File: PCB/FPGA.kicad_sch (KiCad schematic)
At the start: 1 part, among them U1 LFE5U-25F-6BG256C

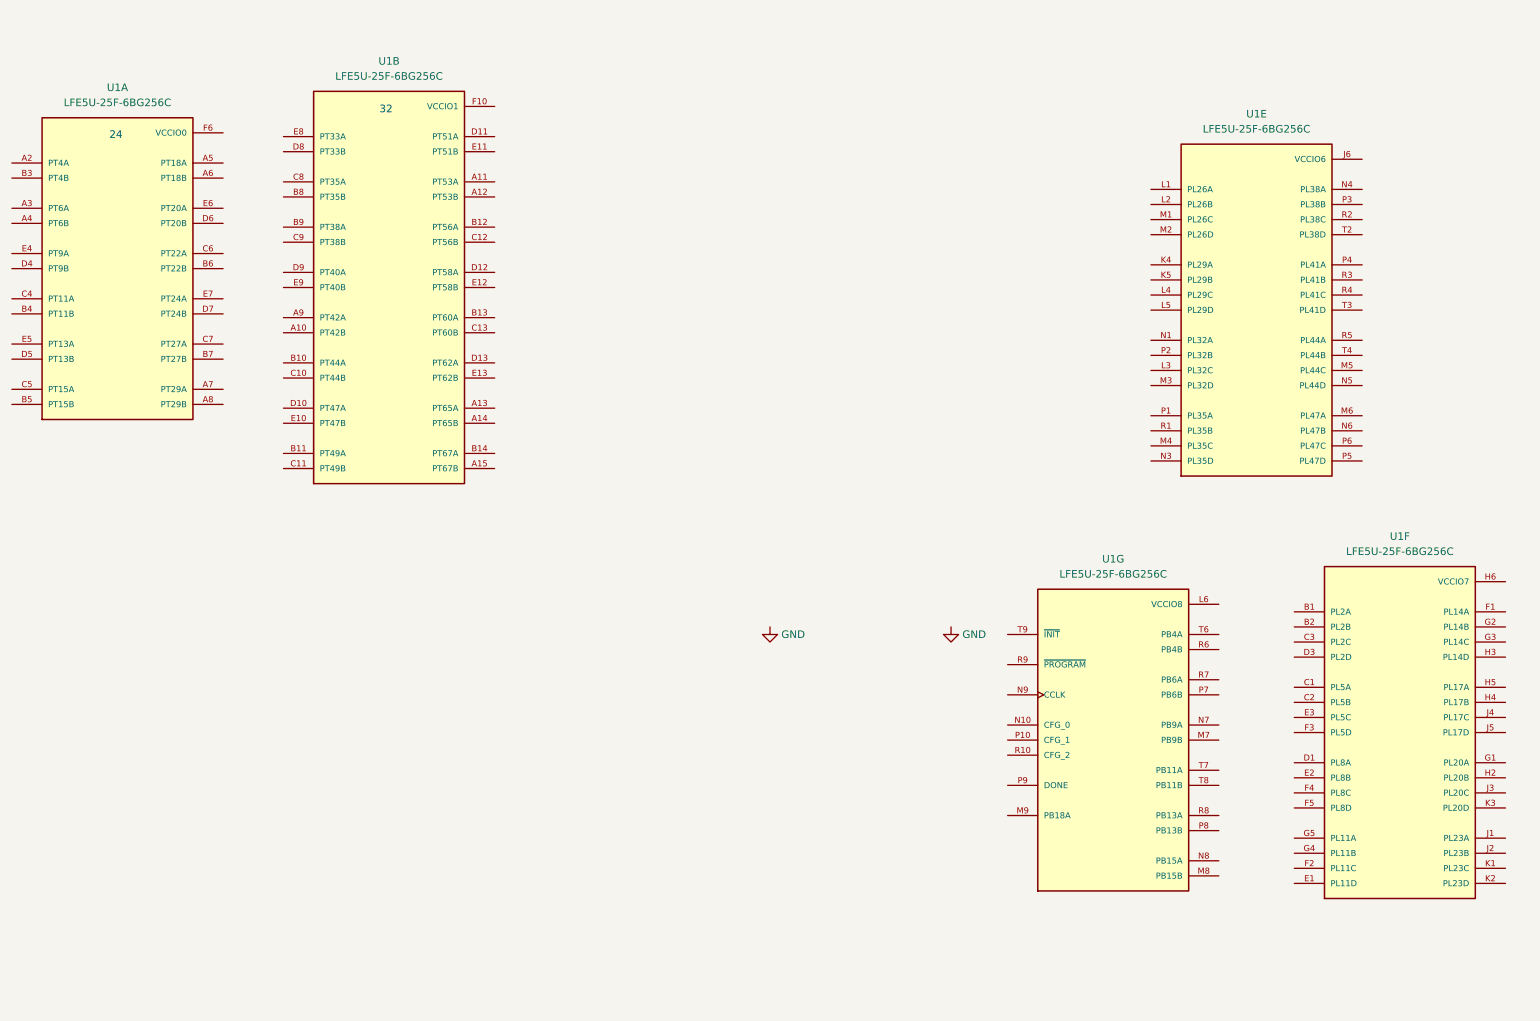
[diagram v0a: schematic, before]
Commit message: route-out in progress
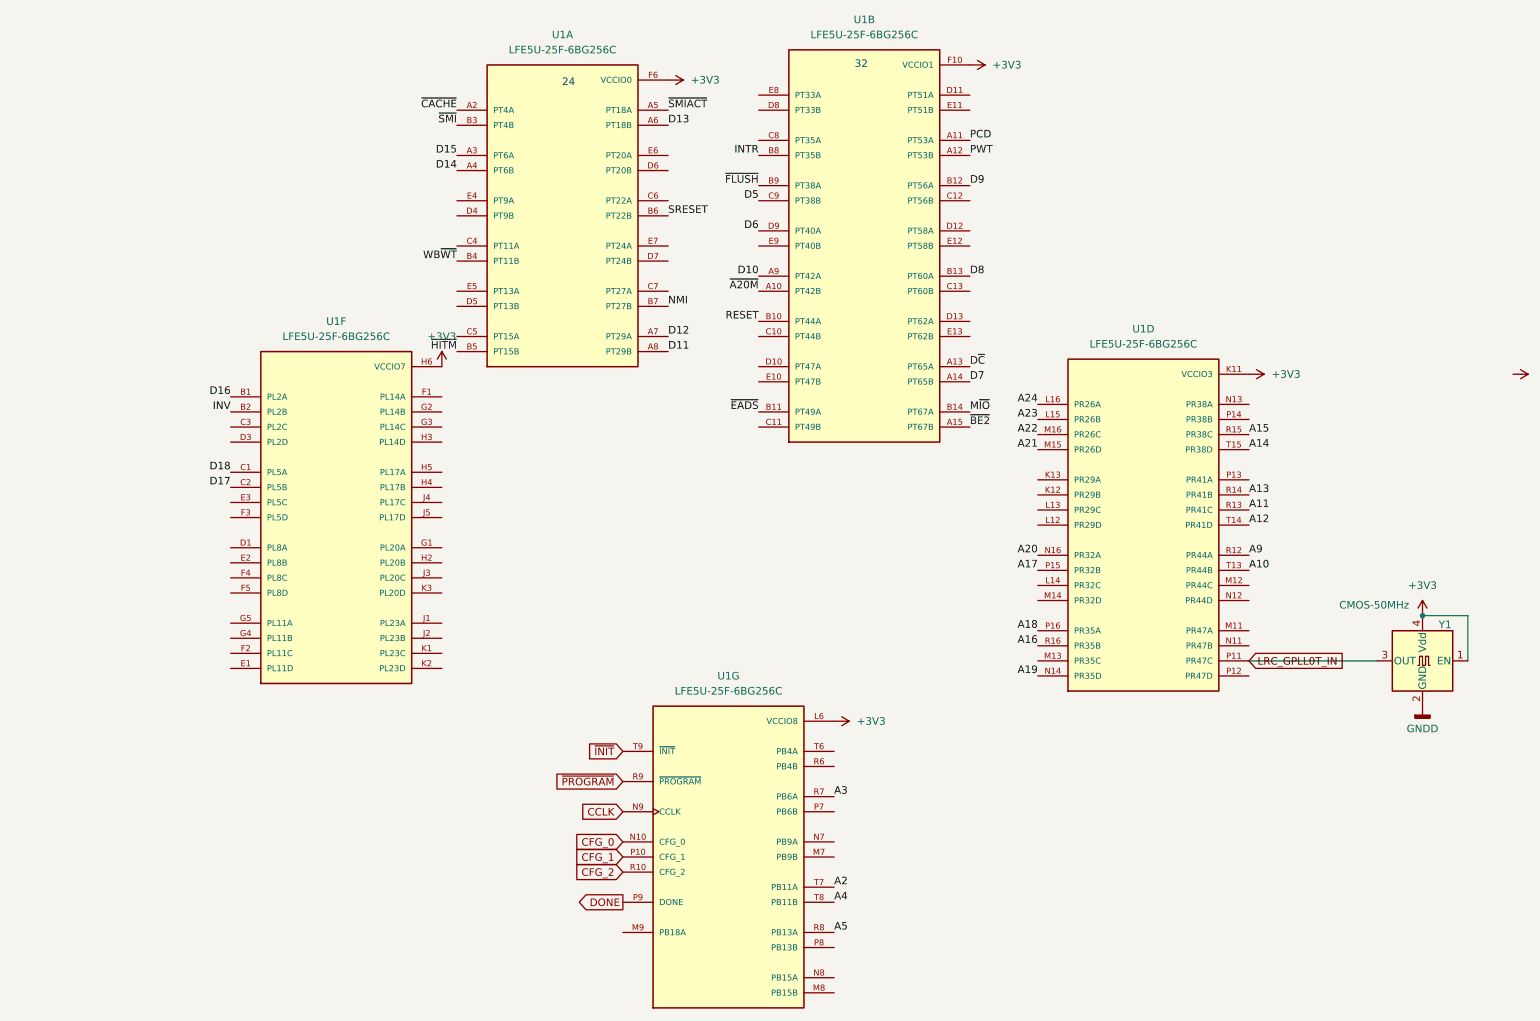
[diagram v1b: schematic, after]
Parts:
- removed unit 5 of U1
- added unit 4 of U1
- added Y1: CMOS-50MHz, Oscillator:Oscillator_SMD_Abracon_ASE-4Pin_3.2x2.5mm, symbol Oscillator:ASE-xxxMHz
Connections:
- net VCCIO0 is gone; now on net +3V3: U1.F6 (VCCIO0), U1.F7 (VCCIO0)
- net VCCIO1 is gone; now on net +3V3: U1.F10 (VCCIO1), U1.F11 (VCCIO1)
- net VCCIO7 is gone; now on net +3V3: U1.H6 (VCCIO7), U1.H7 (VCCIO7)
- net ~{CACHE}: now reaches U1.A2 (PT4A)
- net D15: now reaches U1.A3 (PT6A)
- net D14: now reaches U1.A4 (PT6B)
- net ~{SMIACT}: now reaches U1.A5 (PT18A)
- net D13: now reaches U1.A6 (PT18B)
- net D12: now reaches U1.A7 (PT29A)
- net D11: now reaches U1.A8 (PT29B)
- net ~{SMI}: now reaches U1.B3 (PT4B)
- net WB~{WT}: now reaches U1.B4 (PT11B)
- net ~{HITM}: now reaches U1.B5 (PT15B)
- net SRESET: now reaches U1.B6 (PT22B)
- net NMI: now reaches U1.B7 (PT27B)
- net ~{A20M}: now reaches U1.A10 (PT42B)
- net PCD: now reaches U1.A11 (PT53A)
- net PWT: now reaches U1.A12 (PT53B)
- net D~{C}: now reaches U1.A13 (PT65A)
- net D7: now reaches U1.A14 (PT65B)
- net ~{BE2}: now reaches U1.A15 (PT67B)
- net D10: now reaches U1.A9 (PT42A)
- net RESET: now reaches U1.B10 (PT44A)
- net ~{EADS}: now reaches U1.B11 (PT49A)
- net D9: now reaches U1.B12 (PT56A)
- net D8: now reaches U1.B13 (PT60A)
- net M~{IO}: now reaches U1.B14 (PT67A)
- net INTR: now reaches U1.B8 (PT35B)
- net ~{FLUSH}: now reaches U1.B9 (PT38A)
- net D5: now reaches U1.C9 (PT38B)
- net D6: now reaches U1.D9 (PT40A)
- net +3V3: now reaches U1.L6 (VCCIO8)
- net +3V3: now also U1.K11 (VCCIO3), U1.L11 (VCCIO3), Y1.1 (EN), Y1.4 (Vdd)
- net CFG_0: now reaches U1.N10 (CFG_0)
- net CCLK: now reaches U1.N9 (CCLK)
- net CFG_1: now reaches U1.P10 (CFG_1)
- net DONE: now reaches U1.P9 (DONE)
- net CFG_2: now reaches U1.R10 (CFG_2)
- net A3: now reaches U1.R7 (PB6A)
- net A5: now reaches U1.R8 (PB13A)
- net ~{PROGRAM}: now reaches U1.R9 (~{PROGRAM})
- net A2: now reaches U1.T7 (PB11A)
- net A4: now reaches U1.T8 (PB11B)
- net ~{INIT}: now reaches U1.T9 (~{INIT})
- net D16: now reaches U1.B1 (PL2A)
- net INV: now reaches U1.B2 (PL2B)
- net D18: now reaches U1.C1 (PL5A)
- net D17: now reaches U1.C2 (PL5B)
- new net A10: U1.T13 (PR44B)
- new net A11: U1.R13 (PR41C)
- new net A12: U1.T14 (PR41D)
- new net A13: U1.R14 (PR41B)
- new net A14: U1.T15 (PR38D)
- new net A15: U1.R15 (PR38C)
- new net A16: U1.R16 (PR35B)
- new net A17: U1.P15 (PR32B)
- new net A18: U1.P16 (PR35A)
- new net A19: U1.N14 (PR35D)
- new net A20: U1.N16 (PR32A)
- new net A21: U1.M15 (PR26D)
- new net A22: U1.M16 (PR26C)
- new net A23: U1.L15 (PR26B)
- new net A24: U1.L16 (PR26A)
- new net A9: U1.R12 (PR44A)
- new net GNDD: Y1.2 (GND)
- new net LRC_GPLL0T_IN: U1.P11 (PR47C), Y1.3 (OUT)
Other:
- moved on the sheet: U1B, U1G
